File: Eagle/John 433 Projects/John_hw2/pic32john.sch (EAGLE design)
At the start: 26 parts

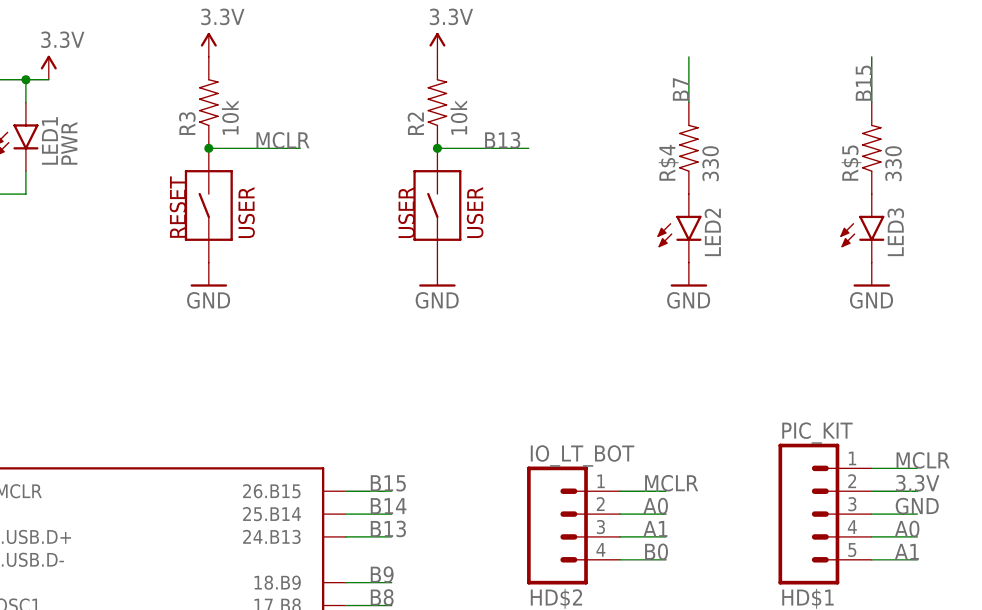
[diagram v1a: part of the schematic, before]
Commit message: draft 1 done and labelled
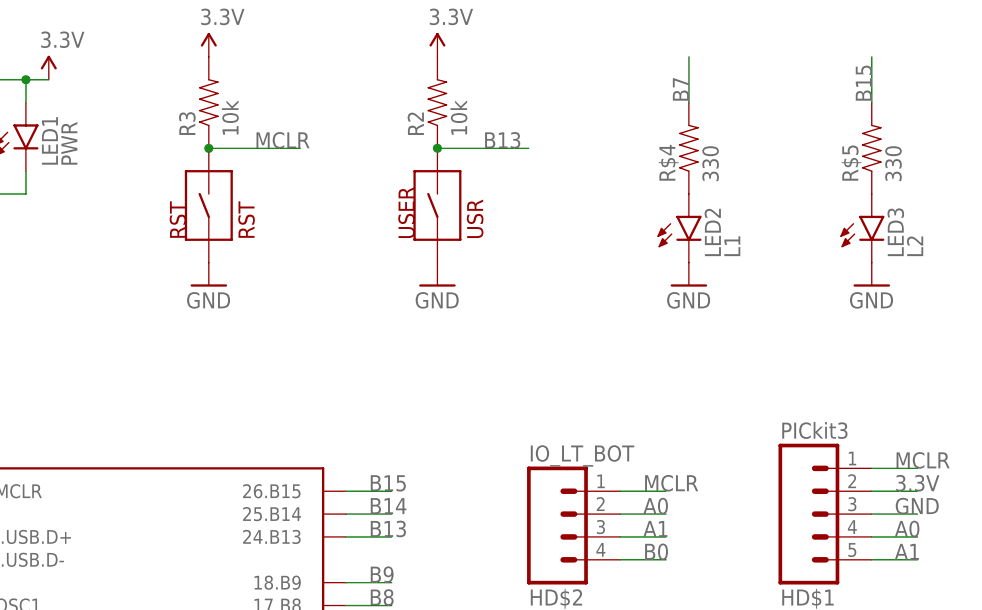
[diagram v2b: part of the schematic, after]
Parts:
- HD$1: value PIC_KIT -> PICkit3
- LED2: value (none) -> L1
- LED3: value (none) -> L2
- RST: value USER -> RST
- USER: value USER -> USR
- renumbered RESET to RST
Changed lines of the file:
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@@
 <grid distance="0.1" unitdist="inch" unit="inch" style="lines" multiple="1" display="no" altdistance="0.01" altunitdist="inch" altunit="inch"/>
 <layers>
-<layer number="1" name="Top" color="4" fill="1" visible="yes" active="no"/>
-<layer number="16" name="Bottom" color="1" fill="1" visible="yes" active="no"/>
-<layer number="17" name="Pads" color="2" fill="1" visible="yes" active="no"/>
-<layer number="18" name="Vias" color="2" fill="1" visible="yes" active="no"/>
-<layer number="19" name="Unrouted" color="6" fill="1" visible="yes" active="no"/>
-<layer number="20" name="Dimension" color="15" fill="1" visible="yes" active="no"/>
-<layer number="21" name="tPlace" color="7" fill="1" visible="yes" active="no"/>
-<layer number="22" name="bPlace" color="7" fill="1" visible="yes" active="no"/>
-<layer number="23" name="tOrigins" color="15" fill="1" visible="yes" active="no"/>
-<layer number="24" name="bOrigins" color="15" fill="1" visible="yes" active="no"/>
-<layer number="25" name="tNames" color="7" fill="1" visible="yes" active="no"/>
-<layer number="26" name="bNames" color="7" fill="1" visible="yes" active="no"/>
-<layer number="27" name="tValues" color="7" fill="1" visible="yes" active="no"/>
-<layer number="28" name="bValues" color="7" fill="1" visible="yes" active="no"/>
+<layer number="1" name="Top" color="4" fill="1" visible="no" active="no"/>
+<layer number="16" name="Bottom" color="1" fill="1" visible="no" active="no"/>
+<layer number="17" name="Pads" color="2" fill="1" visible="no" active="no"/>
+<layer number="18" name="Vias" color="2" fill="1" visible="no" active="no"/>
+<layer number="19" name="Unrouted" color="6" fill="1" visible="no" active="no"/>
+<layer number="20" name="Dimension" color="15" fill="1" visible="no" active="no"/>
+<layer number="21" name="tPlace" color="7" fill="1" visible="no" active="no"/>
+<layer number="22" name="bPlace" color="7" fill="1" visible="no" active="no"/>
+<layer number="23" name="tOrigins" color="15" fill="1" visible="no" active="no"/>
+<layer number="24" name="bOrigins" color="15" fill="1" visible="no" active="no"/>
+<layer number="25" name="tNames" color="7" fill="1" visible="no" active="no"/>
+<layer number="26" name="bNames" color="7" fill="1" visible="no" active="no"/>
+<layer number="27" name="tValues" color="7" fill="1" visible="no" active="no"/>
+<layer number="28" name="bValues" color="7" fill="1" visible="no" active="no"/>
 <layer number="29" name="tStop" color="7" fill="3" visible="no" active="no"/>
 <layer number="30" name="bStop" color="7" fill="6" visible="no" active="no"/>
@@
 <layer number="35" name="tGlue" color="7" fill="4" visible="no" active="no"/>
 <layer number="36" name="bGlue" color="7" fill="5" visible="no" active="no"/>
-<layer number="37" name="tTest" color="7" fill="1" visible="yes" active="no"/>
-<layer number="38" name="bTest" color="7" fill="1" visible="yes" active="no"/>
+<layer number="37" name="tTest" color="7" fill="1" visible="no" active="no"/>
+<layer number="38" name="bTest" color="7" fill="1" visible="no" active="no"/>
 <layer number="39" name="tKeepout" color="4" fill="11" visible="no" active="no"/>
 <layer number="40" name="bKeepout" color="1" fill="11" visible="no" active="no"/>
@@
 <layer number="44" name="Drills" color="7" fill="1" visible="no" active="no"/>
 <layer number="45" name="Holes" color="7" fill="1" visible="no" active="no"/>
-<layer number="46" name="Milling" color="3" fill="1" visible="yes" active="no"/>
-<layer number="47" name="Measures" color="7" fill="1" visible="yes" active="no"/>
-<layer number="48" name="Document" color="7" fill="1" visible="yes" active="no"/>
-<layer number="49" name="Reference" color="7" fill="1" visible="yes" active="no"/>
-<layer number="50" name="dxf" color="7" fill="1" visible="yes" active="no"/>
-<layer number="51" name="tDocu" color="7" fill="1" visible="yes" active="no"/>
-<layer number="52" name="bDocu" color="7" fill="1" visible="yes" active="no"/>
-<layer number="53" name="tGND_GNDA" color="7" fill="9" visible="yes" active="no"/>
-<layer number="54" name="bGND_GNDA" color="1" fill="9" visible="yes" active="no"/>
-<layer number="56" name="wert" color="7" fill="1" visible="yes" active="no"/>
-<layer number="57" name="tCAD" color="7" fill="1" visible="yes" active="no"/>
-<layer number="59" name="tCarbon" color="7" fill="1" visible="yes" active="no"/>
-<layer number="60" name="bCarbon" color="7" fill="1" visible="yes" active="no"/>
+<layer number="46" name="Milling" color="3" fill="1" visible="no" active="no"/>
+<layer number="47" name="Measures" color="7" fill="1" visible="no" active="no"/>
+<layer number="48" name="Document" color="7" fill="1" visible="no" active="no"/>
+<layer number="49" name="Reference" color="7" fill="1" visible="no" active="no"/>
+<layer number="50" name="dxf" color="7" fill="1" visible="no" active="no"/>
+<layer number="51" name="tDocu" color="7" fill="1" visible="no" active="no"/>
+<layer number="52" name="bDocu" color="7" fill="1" visible="no" active="no"/>
+<layer number="53" name="tGND_GNDA" color="7" fill="9" visible="no" active="no"/>
+<layer number="54" name="bGND_GNDA" color="1" fill="9" visible="no" active="no"/>
+<layer number="56" name="wert" color="7" fill="1" visible="no" active="no"/>
+<layer number="57" name="tCAD" color="7" fill="1" visible="no" active="no"/>
+<layer number="59" name="tCarbon" color="7" fill="1" visible="no" active="no"/>
+<layer number="60" name="bCarbon" color="7" fill="1" visible="no" active="no"/>
 <layer number="90" name="Modules" color="5" fill="1" visible="yes" active="yes"/>
 <layer number="91" name="Nets" color="2" fill="1" visible="yes" active="yes"/>
@@
 <part name="C9" library="john433" deviceset="CAP" device="PTH" value="0.1uF"/>
 <part name="C10" library="john433" deviceset="CAP" device="PTH" value="0.1uF"/>
-<part name="HD$1" library="SparkFun-Connectors" deviceset="M05" device="PTH" value="PIC_KIT"/>
+<part name="HD$1" library="SparkFun-Connectors" deviceset="M05" device="PTH" value="PICkit3"/>
 <part name="HD$4" library="SparkFun-Connectors" deviceset="M04" device="PTH" value="IO_LT_BOT"/>
 <part name="HD$3" library="SparkFun-Connectors" deviceset="M04" device="PTH" value="IO_LT_BOT"/>
@@
 <part name="HD$6" library="SparkFun-Connectors" deviceset="M04" device="PTH" value="IO_LT_BOT"/>
 <part name="HD$5" library="SparkFun-Connectors" deviceset="M04" device="PTH" value="IO_LT_BOT"/>
-<part name="USER" library="john433" deviceset="BTN_P8072" device="" value="USER"/>
+<part name="USER" library="john433" deviceset="BTN_P8072" device="" value="USR"/>
 <part name="GND5" library="john433" deviceset="GND" device=""/>
 <part name="P+3" library="john433" deviceset="3.3V" device=""/>
 <part name="R3" library="john433" deviceset="RESISTOR" device="PTH-1/4W" value="10k"/>
-<part name="RESET" library="john433" deviceset="BTN_P8072" device="" value="USER"/>
+<part name="RST" library="john433" deviceset="BTN_P8072" device="" value="RST"/>
 <part name="GND6" library="john433" deviceset="GND" device=""/>
 <part name="P+4" library="john433" deviceset="3.3V" device=""/>
-<part name="LED2" library="john433" deviceset="LED" device="3MM"/>
+<part name="LED2" library="john433" deviceset="LED" device="3MM" value="L1"/>
 <part name="R$4" library="john433" deviceset="RESISTOR" device="PTH-1/4W" value="330"/>
 <part name="GND7" library="john433" deviceset="GND" device=""/>
-<part name="LED3" library="john433" deviceset="LED" device="3MM"/>
+<part name="LED3" library="john433" deviceset="LED" device="3MM" value="L2"/>
 <part name="R$5" library="john433" deviceset="RESISTOR" device="PTH-1/4W" value="330"/>
 <part name="GND8" library="john433" deviceset="GND" device=""/>
@@
 <instance part="P+3" gate="G$1" x="53.34" y="96.52"/>
 <instance part="R3" gate="G$1" x="27.94" y="91.44" rot="R90"/>
-<instance part="RESET" gate="G$1" x="30.48" y="76.2" rot="R90"/>
+<instance part="RST" gate="G$1" x="30.48" y="76.2" rot="R90"/>
 <instance part="GND6" gate="1" x="27.94" y="71.12"/>
 <instance part="P+4" gate="G$1" x="27.94" y="96.52"/>
@@
 </segment>
 <segment>
-<pinref part="RESET" gate="G$1" pin="P$1"/>
+<pinref part="RST" gate="G$1" pin="P$1"/>
 <pinref part="GND6" gate="1" pin="GND"/>
 </segment>
@@
 <segment>
 <pinref part="R3" gate="G$1" pin="1"/>
-<pinref part="RESET" gate="G$1" pin="P$2"/>
+<pinref part="RST" gate="G$1" pin="P$2"/>
 <wire x1="27.94" y1="86.36" x2="38.1" y2="86.36" width="0.1524" layer="91"/>
 <junction x="27.94" y="86.36"/>
